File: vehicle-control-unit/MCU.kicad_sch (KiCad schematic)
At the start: 93 parts, among them J5 FTSH-107-01-F-DV-K-P-TR, Q10 AO3400A, Q12 AO3400A, Q7 AO3400A, Q8 AO3400A, Q9 AO3400A, SW4 PV1H240BB, SW6 Y97KT23B5NAFP, U17 PST360G2-2AA-C0123-ERA040-05K, U18 PST360G2-2AA-C0123-ERA040-05K, U19 PST360G2-2AA-C0123-ERA040-05K, U20 STM32G473RCTx, U21 ISO1044BD, U22 ISO1044BD, U24 MCP6004, U26 STLINK-V3MODS, U31 104990302, Y2 ECS-240-8-37B-CKY-TR

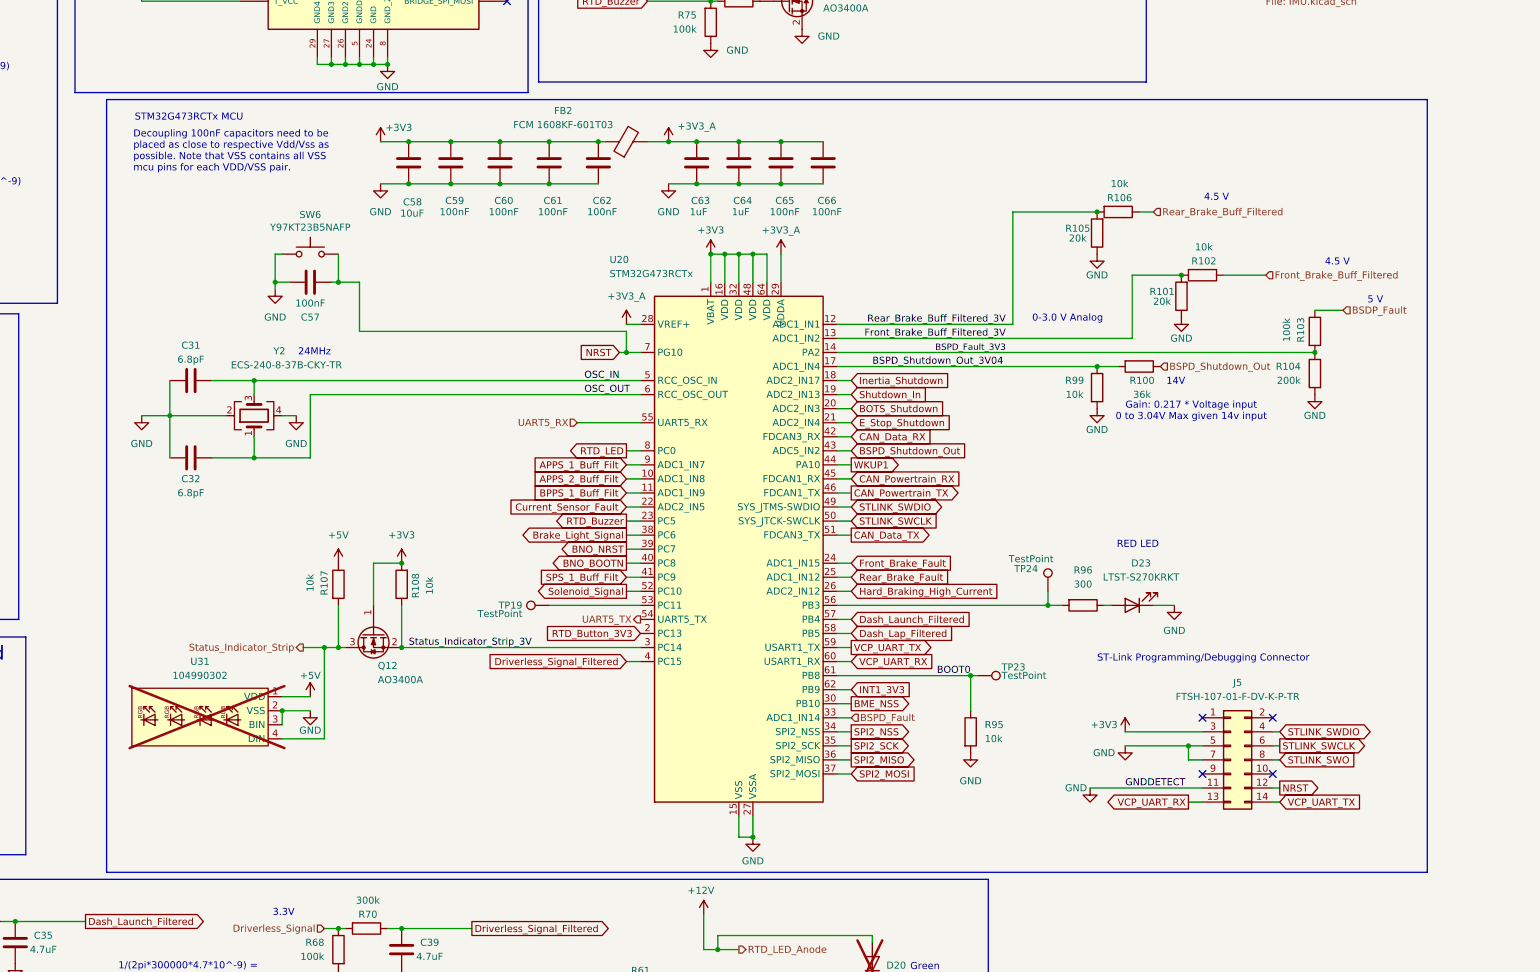
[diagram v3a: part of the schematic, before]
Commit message: added lamp check and removed imu pins
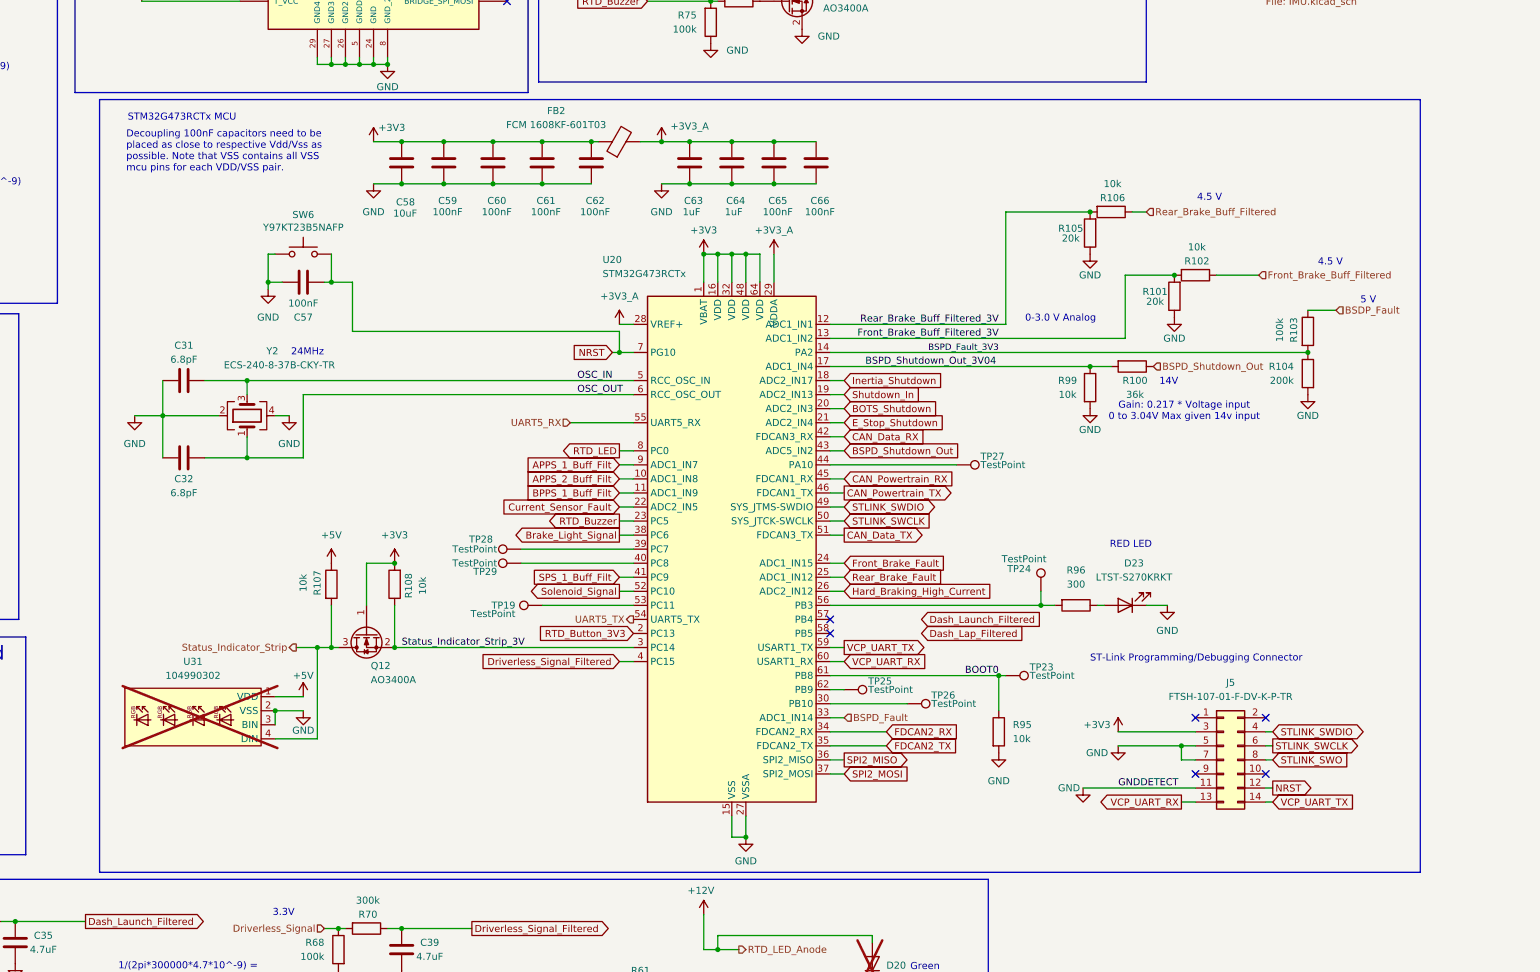
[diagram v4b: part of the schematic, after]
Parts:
- added TP25, TP26, TP27, TP28, TP29: TestPoint, TestPoint:TestPoint_Pad_D1.0mm, symbol Connector:TestPoint
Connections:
- net BME_NSS: no longer U20.30 (PB10)
- net BNO_BOOTN: no longer U20.40 (PC8)
- net BNO_NRST: no longer U20.39 (PC7)
- net Dash_Lap_Filtered: no longer U20.58 (PB5)
- net Dash_Launch_Filtered: no longer U20.57 (PB4)
- net INT1_3V3: no longer U20.62 (PB9)
- net SPI2_NSS: no longer U20.34 (PB12)
- net SPI2_SCK: no longer U20.35 (PB13)
- net WKUP1: no longer U20.44 (PA10)
- new net: TP26.1, U20.30 (PB10)
- new net: TP28.1, U20.39 (PC7)
- new net: TP29.1, U20.40 (PC8)
- new net: TP27.1, U20.44 (PA10)
- new net: TP25.1, U20.62 (PB9)
- new net FDCAN2_RX: U20.34 (PB12)
- new net FDCAN2_TX: U20.35 (PB13)
- no-connect marks 32 -> 34
